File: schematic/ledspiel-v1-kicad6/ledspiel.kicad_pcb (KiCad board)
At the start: 2 copper layers, 90 x 56 mm, 160 parts, among them J1 Keys, J2 SWD Debug, J3 USART Debug, J5 USB_C_Receptacle_USB2.0, J70 Micro_SD_Card_Det, J80 Battery, Q10 BSS138, Q11 BSS138, Q12 BSS138, Q13 BSS138, Q14 BSS138, Q60 SFH300-3/4, Q70 IRLML6402, Q80 BSS138, Q81 IRLML6402, Q82 BSS138, U1 STM32F405RGTx, U100 LM4861, U2 USBLC6-2SC6, U60 TSOP312xx, U80 MCP1640CH, U81 LP38693MP-3.3, Y1 8MHz, Y2 32768Hz

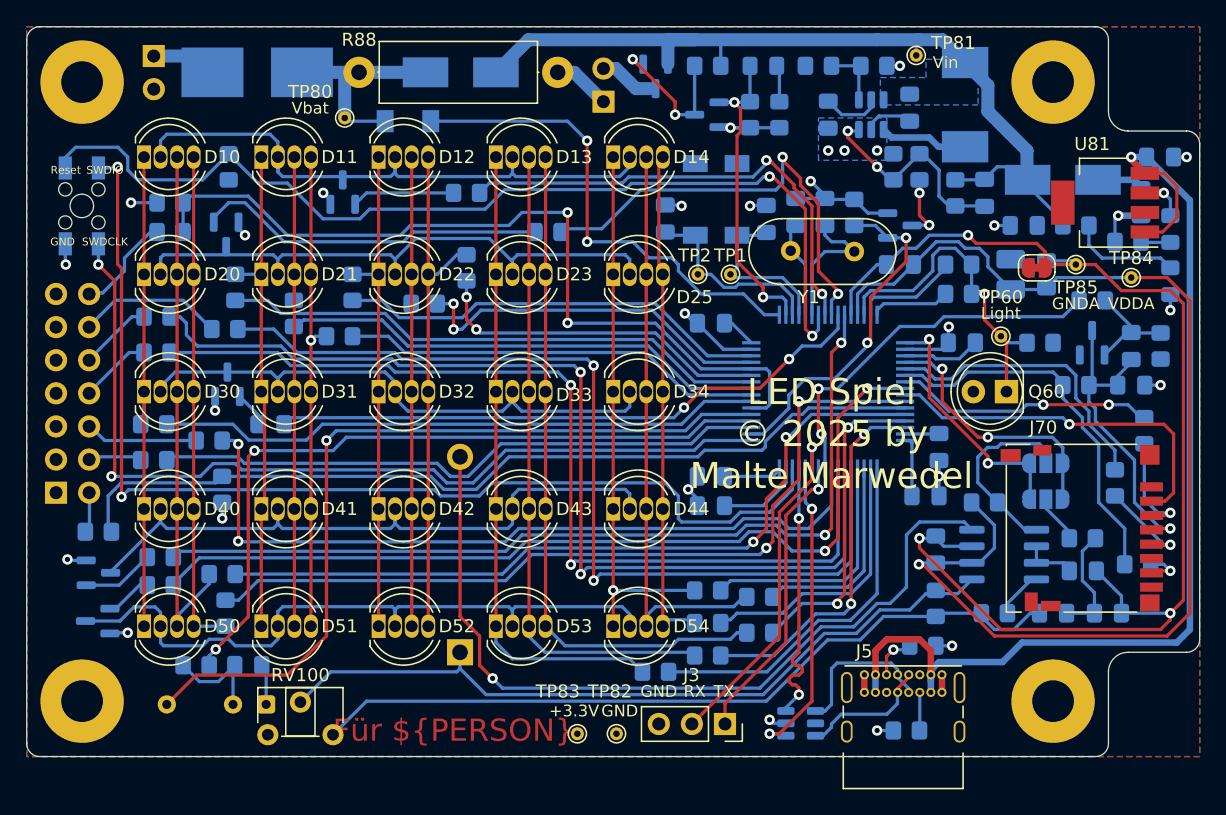
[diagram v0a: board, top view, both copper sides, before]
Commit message: WIP
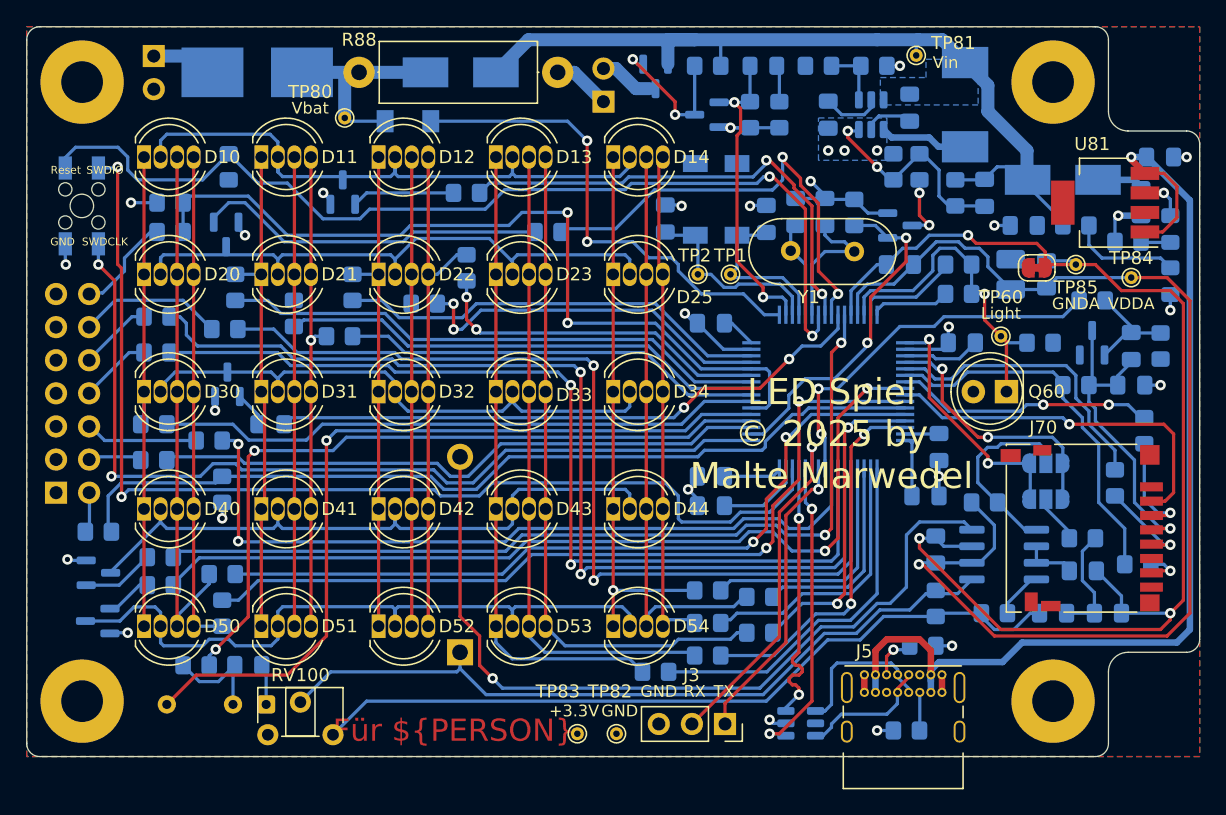
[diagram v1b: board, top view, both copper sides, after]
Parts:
- R102, R110, R111, R112, R113, R114, R115, R116, R30, R31, R32, R33, R34, R60, R70, R91: value 200Ω -> 220Ω
- R103: value 25kΩ -> 27kΩ
- moved R10 0.25 mm to (115.0, 145.0)
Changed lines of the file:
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@@
       (effects (font (size 1 1) (thickness 0.15)) (justify mirror))
     )
-    (fp_text value "200Ω" (at 0 -1.65) (layer "B.Fab")
+    (fp_text value "220Ω" (at 0 -1.65) (layer "B.Fab")
       (effects (font (size 1 1) (thickness 0.15)) (justify mirror))
     )
@@
       (effects (font (size 1 1) (thickness 0.15)) (justify mirror))
     )
-    (fp_text value "200Ω" (at 0 -1.65) (layer "B.Fab")
+    (fp_text value "220Ω" (at 0 -1.65) (layer "B.Fab")
       (effects (font (size 1 1) (thickness 0.15)) (justify mirror))
     )
@@
       (effects (font (size 1 1) (thickness 0.15)) (justify mirror))
     )
-    (fp_text value "200Ω" (at 0 -1.65) (layer "B.Fab")
+    (fp_text value "220Ω" (at 0 -1.65) (layer "B.Fab")
       (effects (font (size 1 1) (thickness 0.15)) (justify mirror))
     )
@@
       (effects (font (size 1 1) (thickness 0.15)) (justify mirror))
     )
-    (fp_text value "200Ω" (at 0 -1.65) (layer "B.Fab")
+    (fp_text value "220Ω" (at 0 -1.65) (layer "B.Fab")
       (effects (font (size 1 1) (thickness 0.15)) (justify mirror))
     )
@@
       (effects (font (size 1 1) (thickness 0.15)) (justify mirror))
     )
-    (fp_text value "200Ω" (at 0 -1.65) (layer "B.Fab")
+    (fp_text value "220Ω" (at 0 -1.65) (layer "B.Fab")
       (effects (font (size 1 1) (thickness 0.15)) (justify mirror))
     )
@@
       (effects (font (size 1 1) (thickness 0.15)) (justify mirror))
     )
-    (fp_text value "25kΩ" (at 0 -1.65 90) (layer "B.Fab")
+    (fp_text value "27kΩ" (at 0 -1.65 90) (layer "B.Fab")
       (effects (font (size 1 1) (thickness 0.15)) (justify mirror))
     )
@@
       (effects (font (size 1 1) (thickness 0.15)) (justify mirror))
     )
-    (fp_text value "200Ω" (at 0 -1.65) (layer "B.Fab")
+    (fp_text value "220Ω" (at 0 -1.65) (layer "B.Fab")
       (effects (font (size 1 1) (thickness 0.15)) (justify mirror))
     )
@@
       (effects (font (size 1 1) (thickness 0.15)) (justify mirror))
     )
-    (fp_text value "200Ω" (at 0 -1.65) (layer "B.Fab")
+    (fp_text value "220Ω" (at 0 -1.65) (layer "B.Fab")
       (effects (font (size 1 1) (thickness 0.15)) (justify mirror))
     )
@@
       (effects (font (size 0.9 0.9) (thickness 0.15)) (justify mirror))
     )
-    (fp_text value "200Ω" (at 0 -1.65) (layer "B.Fab")
+    (fp_text value "220Ω" (at 0 -1.65) (layer "B.Fab")
       (effects (font (size 1 1) (thickness 0.15)) (justify mirror))
     )
@@
       (effects (font (size 1 1) (thickness 0.15)) (justify mirror))
     )
-    (fp_text value "200Ω" (at 0 -1.65) (layer "B.Fab")
+    (fp_text value "220Ω" (at 0 -1.65) (layer "B.Fab")
       (effects (font (size 1 1) (thickness 0.15)) (justify mirror))
     )
@@
       (effects (font (size 1 1) (thickness 0.15)) (justify mirror))
     )
-    (fp_text value "200Ω" (at 0 -1.65) (layer "B.Fab")
+    (fp_text value "220Ω" (at 0 -1.65) (layer "B.Fab")
       (effects (font (size 1 1) (thickness 0.15)) (justify mirror))
     )
@@
       (effects (font (size 1 1) (thickness 0.15)) (justify mirror))
     )
-    (fp_text value "200Ω" (at 0 -1.65) (layer "B.Fab")
+    (fp_text value "220Ω" (at 0 -1.65) (layer "B.Fab")
       (effects (font (size 1 1) (thickness 0.15)) (justify mirror))
     )
@@
       (effects (font (size 1 1) (thickness 0.15)) (justify mirror))
     )
-    (fp_text value "200Ω" (at 0 -1.65) (layer "B.Fab")
+    (fp_text value "220Ω" (at 0 -1.65) (layer "B.Fab")
       (effects (font (size 1 1) (thickness 0.15)) (justify mirror))
     )
@@
       (effects (font (size 1 1) (thickness 0.15)) (justify mirror))
     )
-    (fp_text value "200Ω" (at 0 -1.65) (layer "B.Fab")
+    (fp_text value "220Ω" (at 0 -1.65) (layer "B.Fab")
       (effects (font (size 1 1) (thickness 0.15)) (justify mirror))
     )
@@
       (effects (font (size 1 1) (thickness 0.15)) (justify mirror))
     )
-    (fp_text value "200Ω" (at 0 -1.65) (layer "B.Fab")
+    (fp_text value "220Ω" (at 0 -1.65) (layer "B.Fab")
       (effects (font (size 1 1) (thickness 0.15)) (justify mirror))
     )
@@
       (effects (font (size 1 1) (thickness 0.15)) (justify mirror))
     )
-    (fp_text value "200Ω" (at 0 -1.65 90) (layer "B.Fab")
+    (fp_text value "220Ω" (at 0 -1.65 90) (layer "B.Fab")
       (effects (font (size 1 1) (thickness 0.15)) (justify mirror))
     )
@@
       (effects (font (size 1 1) (thickness 0.15)) (justify mirror))
     )
-    (fp_text value "200Ω" (at 0 -1.65) (layer "B.Fab")
+    (fp_text value "220Ω" (at 0 -1.65) (layer "B.Fab")
       (effects (font (size 1 1) (thickness 0.15)) (justify mirror))
     )
@@
   )
   (footprint "Resistor_SMD:R_0805_2012Metric_Pad1.20x1.40mm_HandSolder" (layer "B.Cu")
-    (at 115.25 145 90)
+    (at 115 145 90)
     (descr "Resistor SMD 0805 (2012 Metric), square (rectangular) end terminal, IPC_7351 nominal with elongated pad for handsoldering. (Body size source: IPC-SM-782 page 72, https://www.pcb-3d.com/wordpress/wp-content/uploads/ipc-sm-782a_amendment_1_and_2.pdf), generated with kicad-footprint-generator")
     (tags "resistor handsolder")
@@
   (segment (start 112.81 137) (end 112.81 146) (width 0.25) (layer "F.Cu") (net 22))
   (segment (start 112.81 128) (end 112.81 137) (width 0.25) (layer "F.Cu") (net 22))
-  (segment (start 115.25 146) (end 112.81 146) (width 0.25) (layer "B.Cu") (net 22))
+  (segment (start 115 146) (end 112.81 146) (width 0.25) (layer "B.Cu") (net 22))
   (segment (start 118 146) (end 118 137) (width 0.25) (layer "F.Cu") (net 23))
   (segment (start 118 137) (end 118.25 136.75) (width 0.25) (layer "F.Cu") (net 23))
@@
   (via (at 156.75 140) (size 0.8) (drill 0.4) (layers "F.Cu" "B.Cu") (net 90))
   (via (at 159.25 128.75) (size 0.8) (drill 0.4) (layers "F.Cu" "B.Cu") (net 90))
-  (segment (start 136.75 142.5) (end 117.75 142.5) (width 0.25) (layer "B.Cu") (net 90))
-  (segment (start 156.75 140) (end 156.25 140.5) (width 0.25) (layer "B.Cu") (net 90))
-  (segment (start 156.25 140.5) (end 138.75 140.5) (width 0.25) (layer "B.Cu") (net 90))
-  (segment (start 116.25 144) (end 115.25 144) (width 0.25) (layer "B.Cu") (net 90))
   (segment (start 138.75 140.5) (end 136.75 142.5) (width 0.25) (layer "B.Cu") (net 90))
+  (segment (start 156.75 140) (end 156.25 140.5) (width 0.25) (layer "B.Cu") (net 90))
+  (segment (start 136.75 142.5) (end 117.75 142.5) (width 0.25) (layer "B.Cu") (net 90))
   (segment (start 117.75 142.5) (end 116.25 144) (width 0.25) (layer "B.Cu") (net 90))
+  (segment (start 156.25 140.5) (end 138.75 140.5) (width 0.25) (layer "B.Cu") (net 90))
+  (segment (start 116.25 144) (end 115 144) (width 0.25) (layer "B.Cu") (net 90))
   (segment (start 159.25 128.75) (end 167.4 128.75) (width 0.25) (layer "B.Cu") (net 90))
   (segment (start 156.75 136.25) (end 158.25 134.75) (width 0.25) (layer "F.Cu") (net 91))
@@
   (via (at 162.25 120.5) (size 0.8) (drill 0.4) (layers "F.Cu" "B.Cu") (net 106))
   (via (at 158 110) (size 0.8) (drill 0.4) (layers "F.Cu" "B.Cu") (net 106))
+  (segment (start 158 111.75) (end 157.225 112.525) (width 0.25) (layer "B.Cu") (net 106))
   (segment (start 141.25 115.5) (end 141 115.75) (width 0.25) (layer "B.Cu") (net 106))
-  (segment (start 158 112) (end 157.475 112.525) (width 0.25) (layer "B.Cu") (net 106))
+  (segment (start 145.1875 115.5) (end 141.25 115.5) (width 0.25) (layer "B.Cu") (net 106))
   (segment (start 161.75 121) (end 161.75 122.1) (width 0.25) (layer "B.Cu") (net 106))
-  (segment (start 147.1 112.525) (end 144.125 115.5) (width 0.25) (layer "B.Cu") (net 106))
-  (segment (start 144.125 115.5) (end 141.25 115.5) (width 0.25) (layer "B.Cu") (net 106))
   (segment (start 162.25 120.5) (end 161.75 121) (width 0.25) (layer "B.Cu") (net 106))
-  (segment (start 158 110) (end 158 112) (width 0.25) (layer "B.Cu") (net 106))
-  (segment (start 157.475 112.525) (end 147.1 112.525) (width 0.25) (layer "B.Cu") (net 106))
+  (segment (start 157.225 112.525) (end 148.1625 112.525) (width 0.25) (layer "B.Cu") (net 106))
+  (segment (start 148.1625 112.525) (end 145.1875 115.5) (width 0.25) (layer "B.Cu") (net 106))
+  (segment (start 158 110) (end 158 111.75) (width 0.25) (layer "B.Cu") (net 106))
   (segment (start 156.25 127.75) (end 158.5 125.5) (width 0.25) (layer "F.Cu") (net 107))
   (segment (start 150.431694 129.222996) (end 151.90469 127.75) (width 0.25) (layer "F.Cu") (net 107))
